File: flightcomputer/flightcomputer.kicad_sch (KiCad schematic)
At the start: 81 parts, among them J1 Conn_Coaxial, J10 Conn_01x03, J11 Conn_01x03, J12 ESQ-113-14-G-D, J13 Conn_01x07, J2 Conn_Coaxial, J3 Conn_Coaxial, J4 Conn_Coaxial, J5 S3B-PH-K-S-GW, J6 S3B-PH-K-S-GW, J7 S4B-PH-K-S_LF__SN_, J8 S3B-PH-K-S-GW, J9 Conn_01x06, U1 MAX-M10S, U2 LIS2MDLTR, U3 BMI088, U4 MS5607-02BA, U5 ESP32-S3-WROOM-1-N4, U7 Teensy4.1, U8 LSM6DSO32TR, U9 RFM96W-433S2

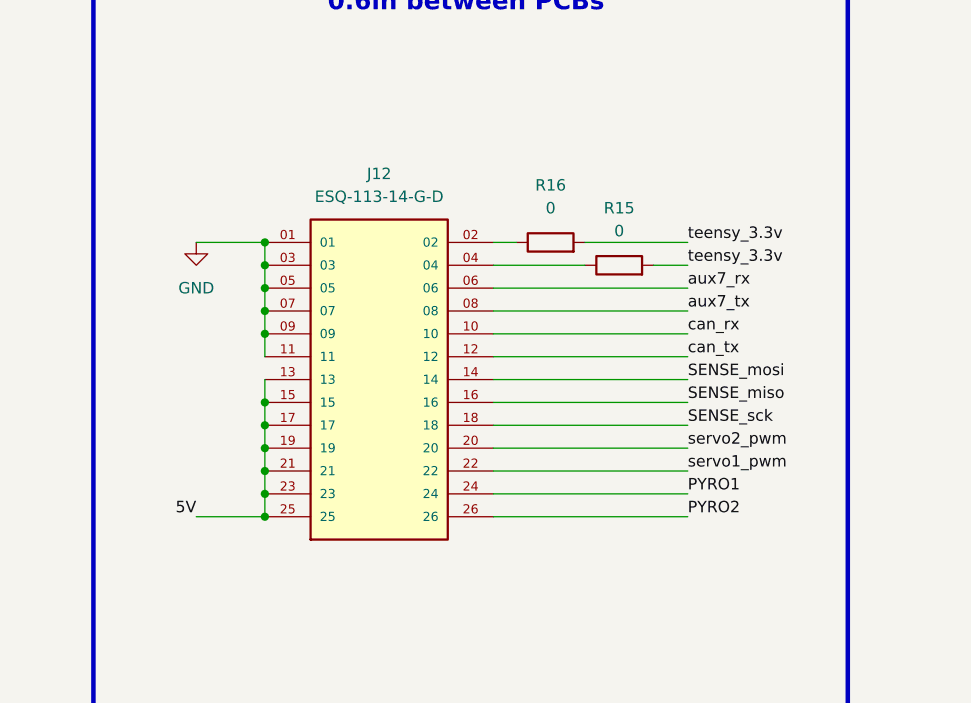
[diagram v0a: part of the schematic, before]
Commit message: resize
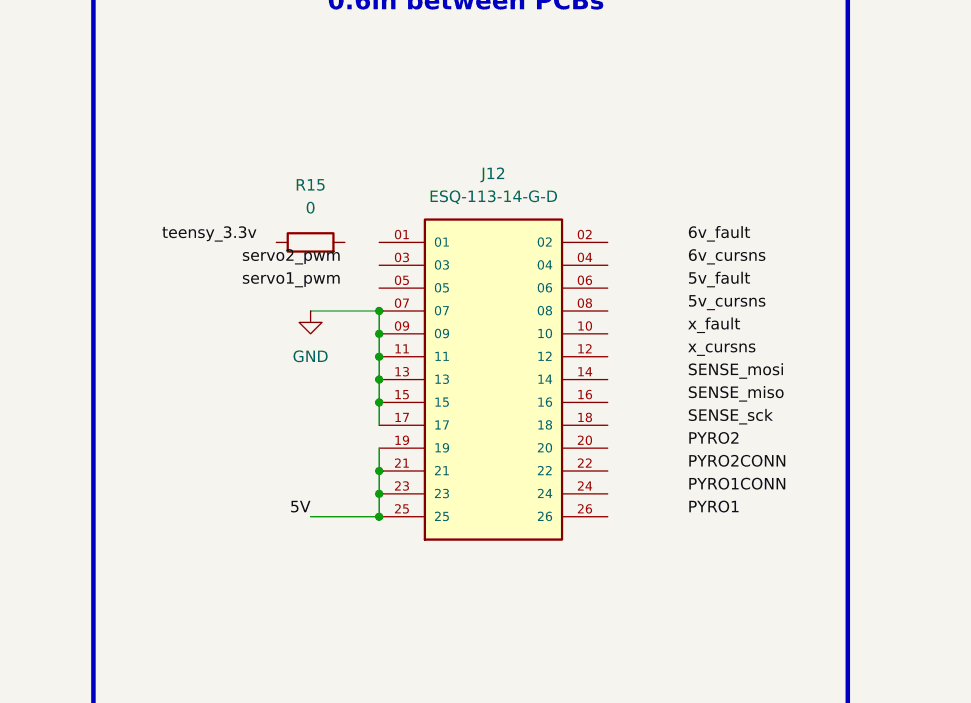
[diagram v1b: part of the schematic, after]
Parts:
- removed R16: 0, Resistor_SMD:R_0603_1608Metric_Pad0.98x0.95mm_HandSolder, symbol Device:R
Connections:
- net 5V: no longer J12.13, J12.15, J12.17
- net GND: now also J12.13, J12.15, J12.17; no longer J12.01, J12.03, J12.05
- net PYRO1: no longer J12.24
- net PYRO2: no longer J12.26
- net SENSE_miso: no longer J12.16
- net SENSE_mosi: no longer J12.14
- net SENSE_sck: no longer J12.18
- net aux7_rx: no longer J12.06
- net aux7_tx: no longer J12.08
- net can_rx: no longer J12.10
- net can_tx: no longer J12.12
- net servo1_pwm: no longer J12.22
- net servo2_pwm: no longer J12.20
- net teensy_3.3v: no longer R15.2
- net at J12.04: no longer R15.1
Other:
- moved on the sheet: J12, R15
